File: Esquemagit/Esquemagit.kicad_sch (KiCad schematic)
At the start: 26 parts, among them U1 LMV321, U2 LM358, U5 ESP32-WROOM-32

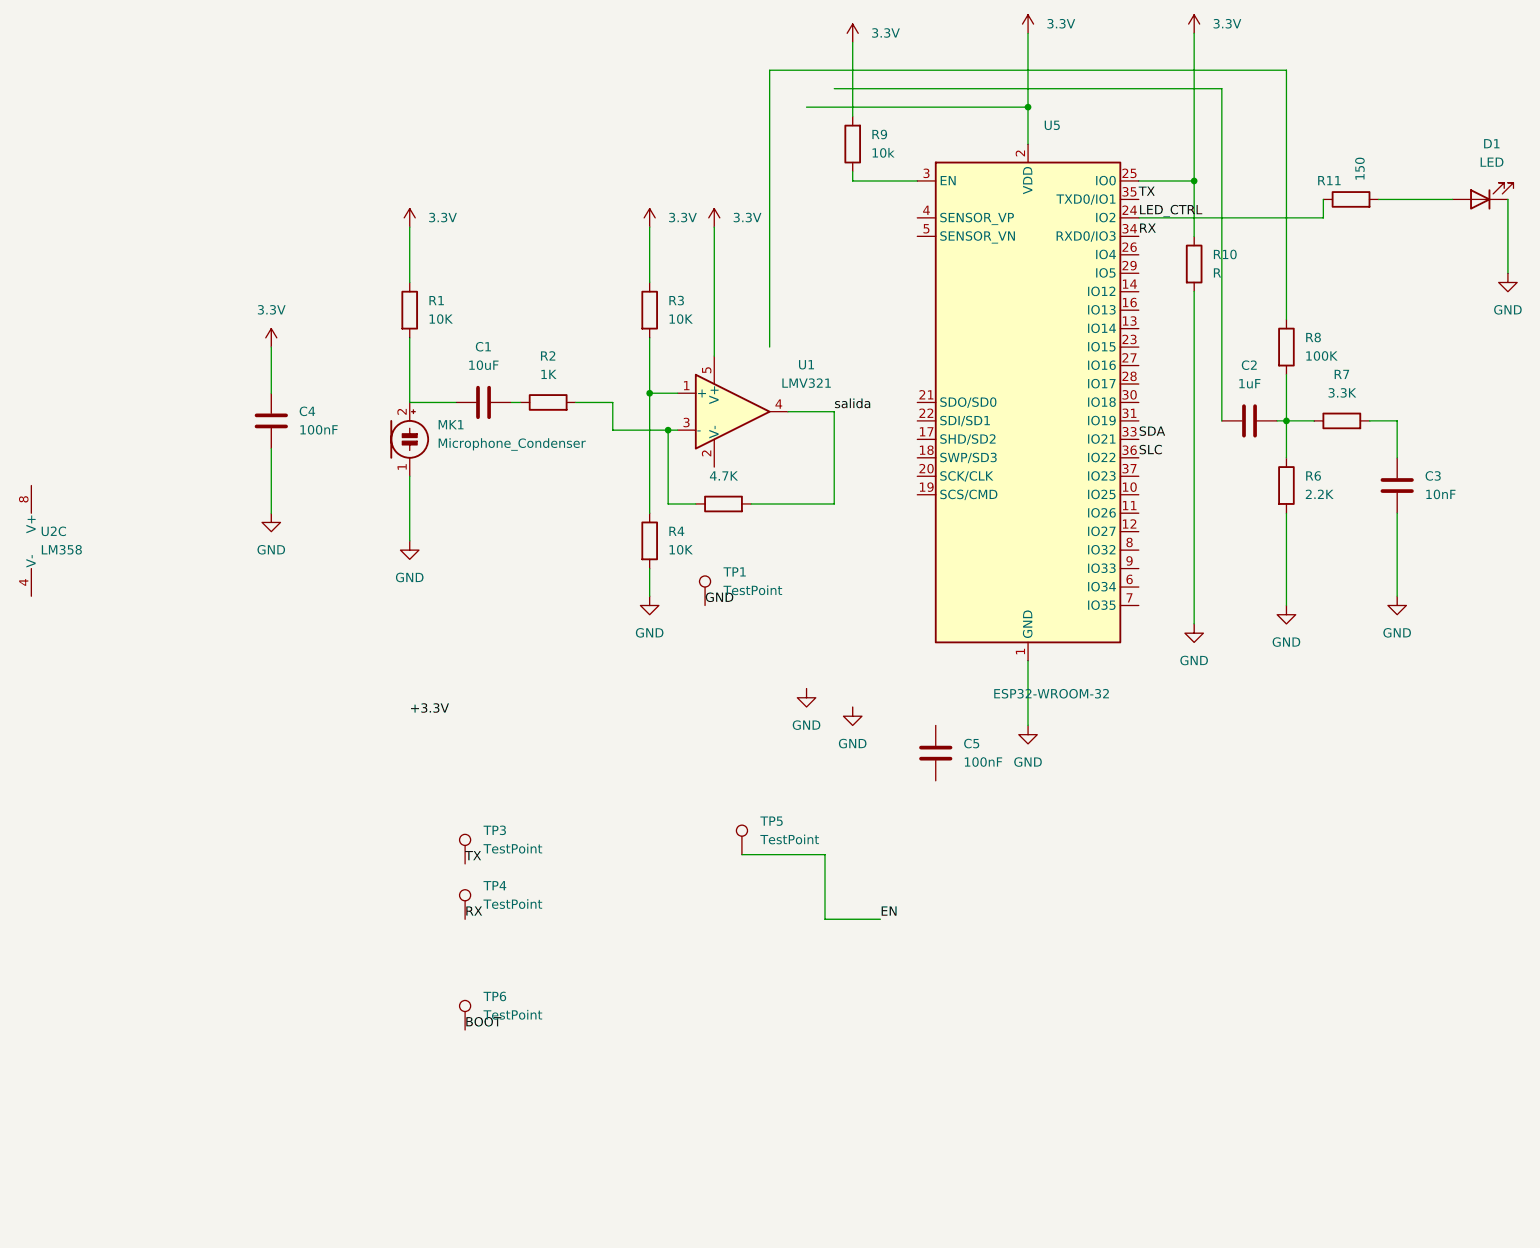
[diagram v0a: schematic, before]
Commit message: feat: actualizaciones en el diseño 2
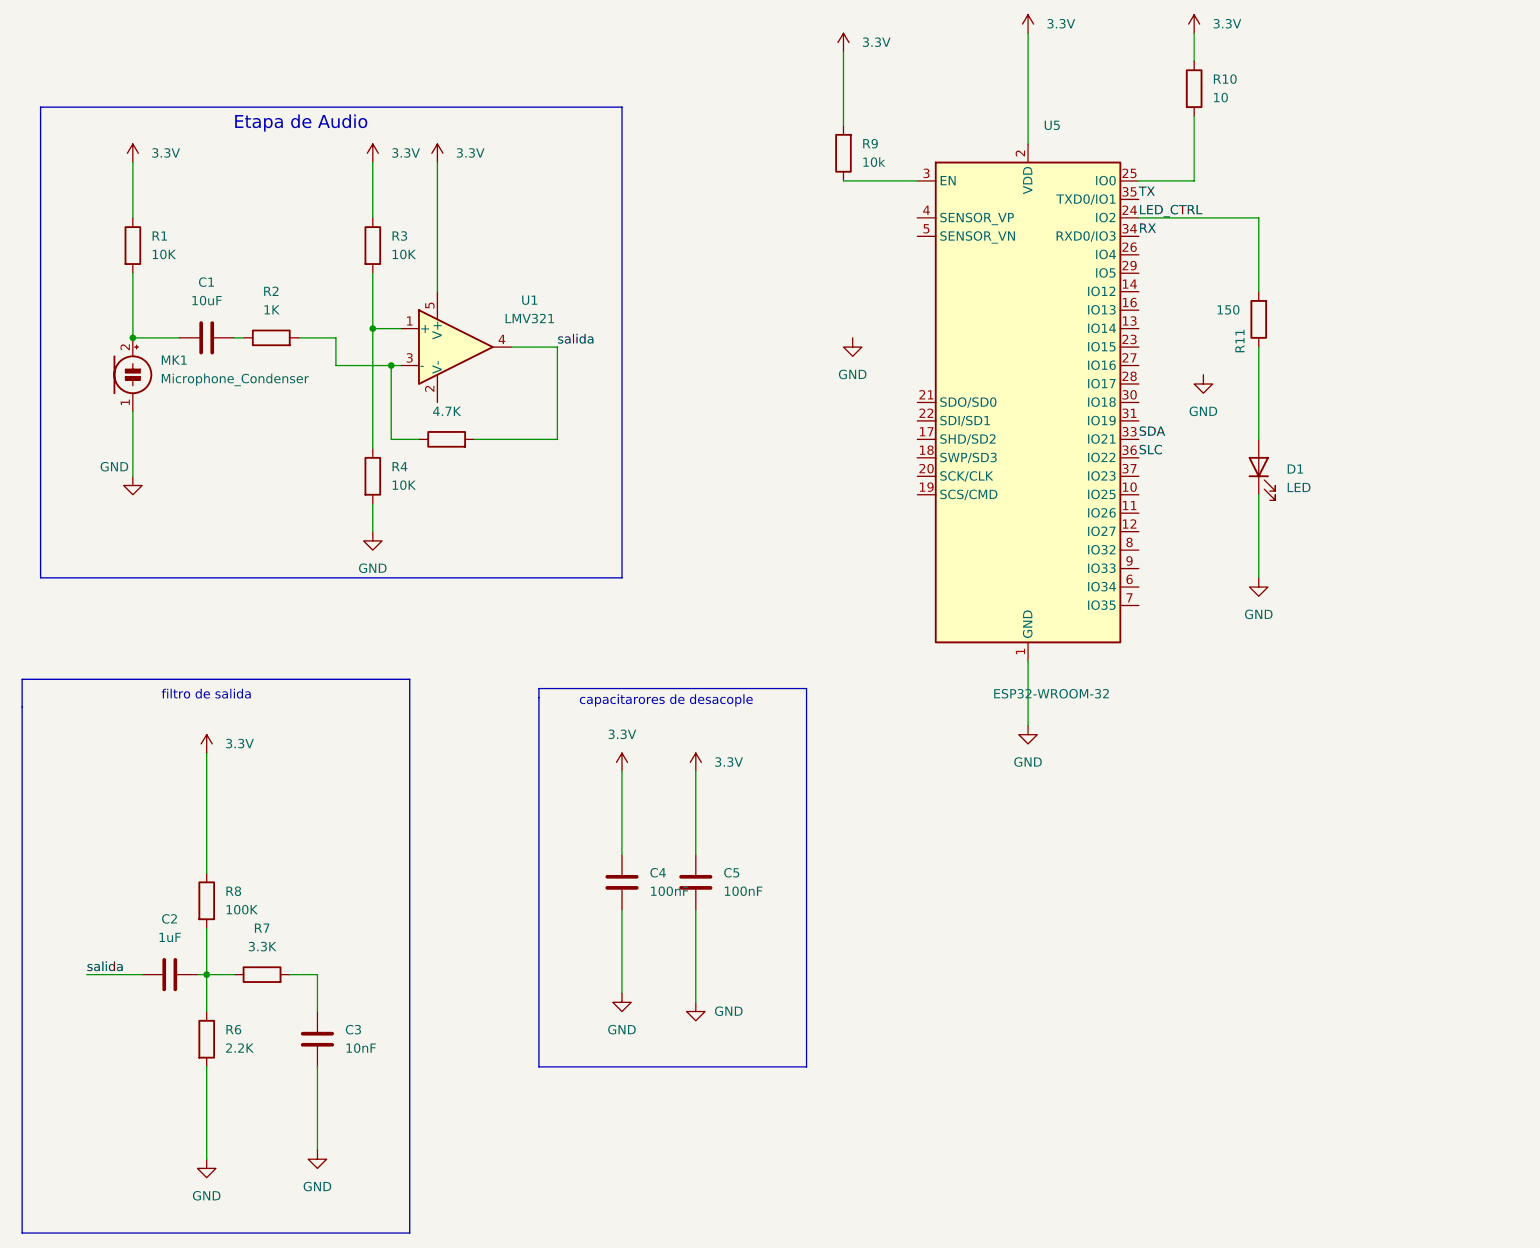
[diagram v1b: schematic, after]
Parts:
- removed TP1, TP3, TP4, TP5, TP6: TestPoint, TestPoint:TestPoint_Loop_D2.54mm_Drill1.5mm_Beaded, symbol Connector:TestPoint
- removed U2: LM358, Package_DIP:DIP-8_W7.62mm_Socket, symbol Amplifier_Operational:LM358
- C2, C3, C5: footprint Capacitor_THT:C_Disc_D5.0mm_W2.5mm_P5.00mm -> Capacitor_SMD:C_0805_2012Metric
- D1: footprint LED_SMD:LED_01005_0402Metric -> LED_SMD:LED_0805_2012Metric
- R10: value R -> 10; footprint Resistor_THT:R_Axial_DIN0207_L6.3mm_D2.5mm_P7.62mm_Horizontal -> Resistor_SMD:R_0805_2012Metric
- R11, R6, R7, R8, R9: footprint Resistor_THT:R_Axial_DIN0207_L6.3mm_D2.5mm_P7.62mm_Horizontal -> Resistor_SMD:R_0805_2012Metric
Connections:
- net 3.3V: now also C5.2, R8.1; no longer U5.25 (IO0)
- net GND: now also C5.1; no longer R10.2
- net LED_CTRL: now also R11.2; no longer R11.1
- net salida: now also C2.1
- net at D1.2 (A): now also R11.1; no longer R11.2
- new net: R10.2, U5.25 (IO0)
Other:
- note added: "Etapa de Audio"
- note added: "capacitarores de desacople"
- note added: "filtro de salida"
- moved on the sheet: C1, C2, C3, C4, C5, D1, MK1, R1, R10, R11, R2, R3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
